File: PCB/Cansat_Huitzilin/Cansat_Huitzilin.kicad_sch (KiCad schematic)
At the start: 72 parts, among them IC1 AP64501SP-13, IC2 114993390, IC3 BMM350, IC4 BMI323, IC5 STCC4-D-R3, IC6 SHT40-AD1B-R2, J1 Screw_Terminal_01x02, J2 Conn_01x04, J3 Conn_01x03, J4 Conn_01x06, J5 Conn_01x03, J6 503398-1892, J7 Conn_01x04, Q1 NPN, SW1 SW_Wuerth_450301014042, SW2 SW_Push, SW3 SW_Push, U1 ESP32-S3-MINI-1U, U3 BMP581

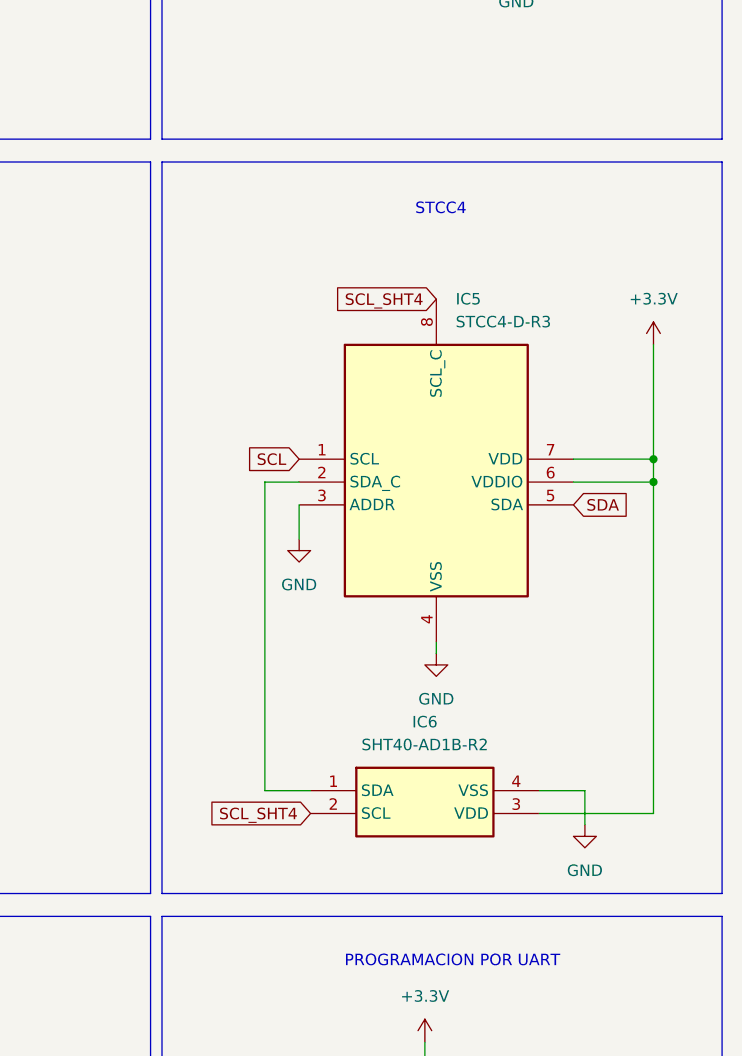
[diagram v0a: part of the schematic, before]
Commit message: save
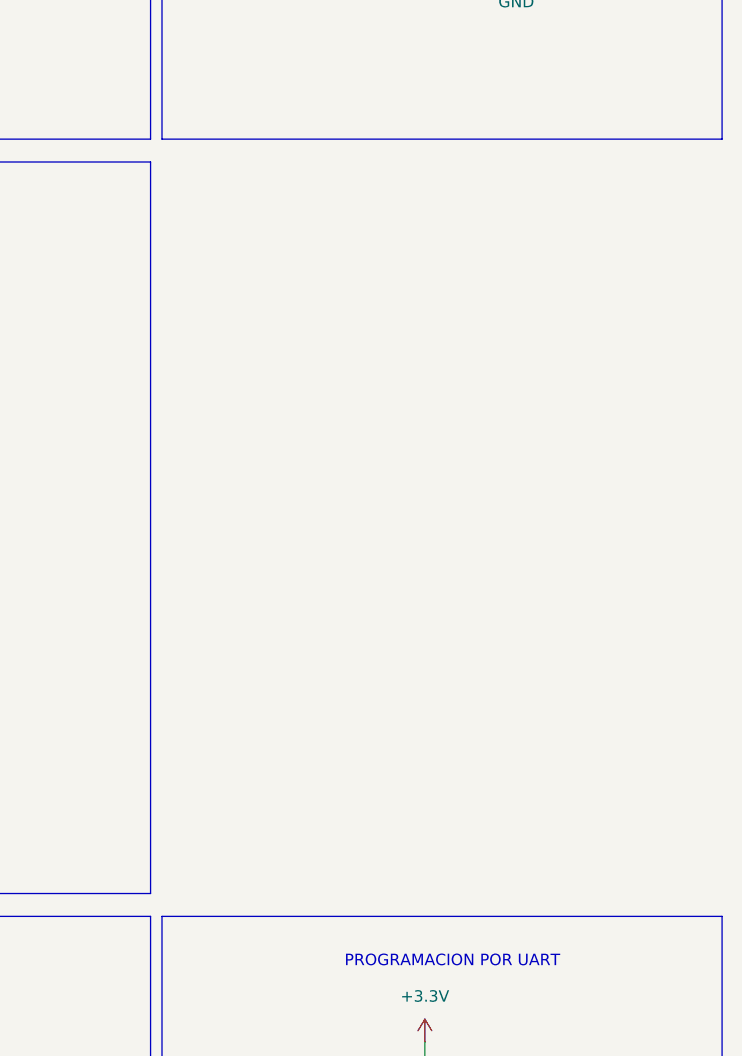
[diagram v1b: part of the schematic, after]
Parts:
- removed IC5: STCC4-D-R3, SamacSys_Parts:STCC4DR3, symbol SamacSys_Parts:STCC4-D-R3
- removed IC6: SHT40-AD1B-R2, SamacSys_Parts:SHT40AD1BR2, symbol SamacSys_Parts:SHT40-AD1B-R2
- H1, H2, H3, H4: footprint MountingHole:MountingHole_3.2mm_M3 -> MountingHole:MountingHole_3.2mm_M3_Pad_Via
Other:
- note removed: "STCC4"
